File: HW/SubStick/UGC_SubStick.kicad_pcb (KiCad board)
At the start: 2 copper layers, 50.1 x 31 mm, 9 parts, among them J1 Conn_01x06_Pin, J2 503480-0640, SW1 GL18_SW, U1 GH39F (Hall SOT23), U2 GH39F (Hall SOT23)

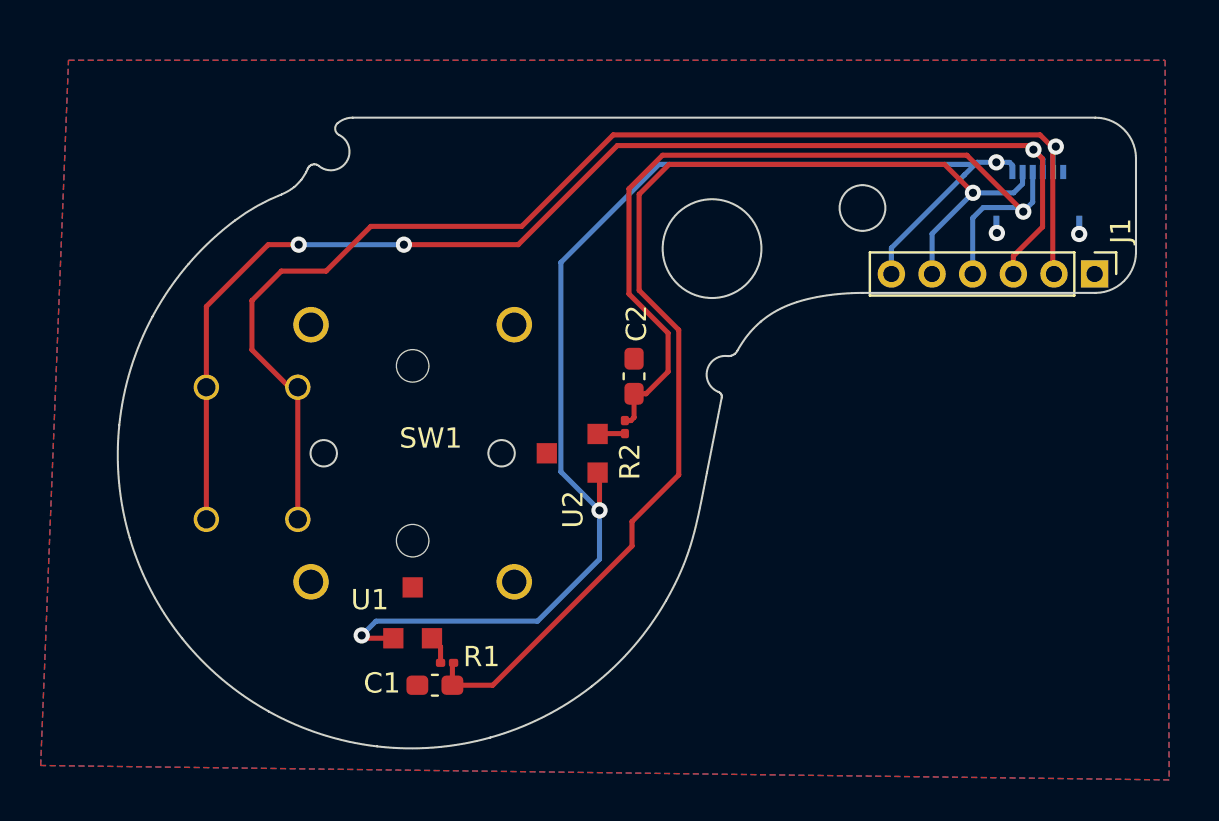
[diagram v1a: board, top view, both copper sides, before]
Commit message: R4 updates to hardware
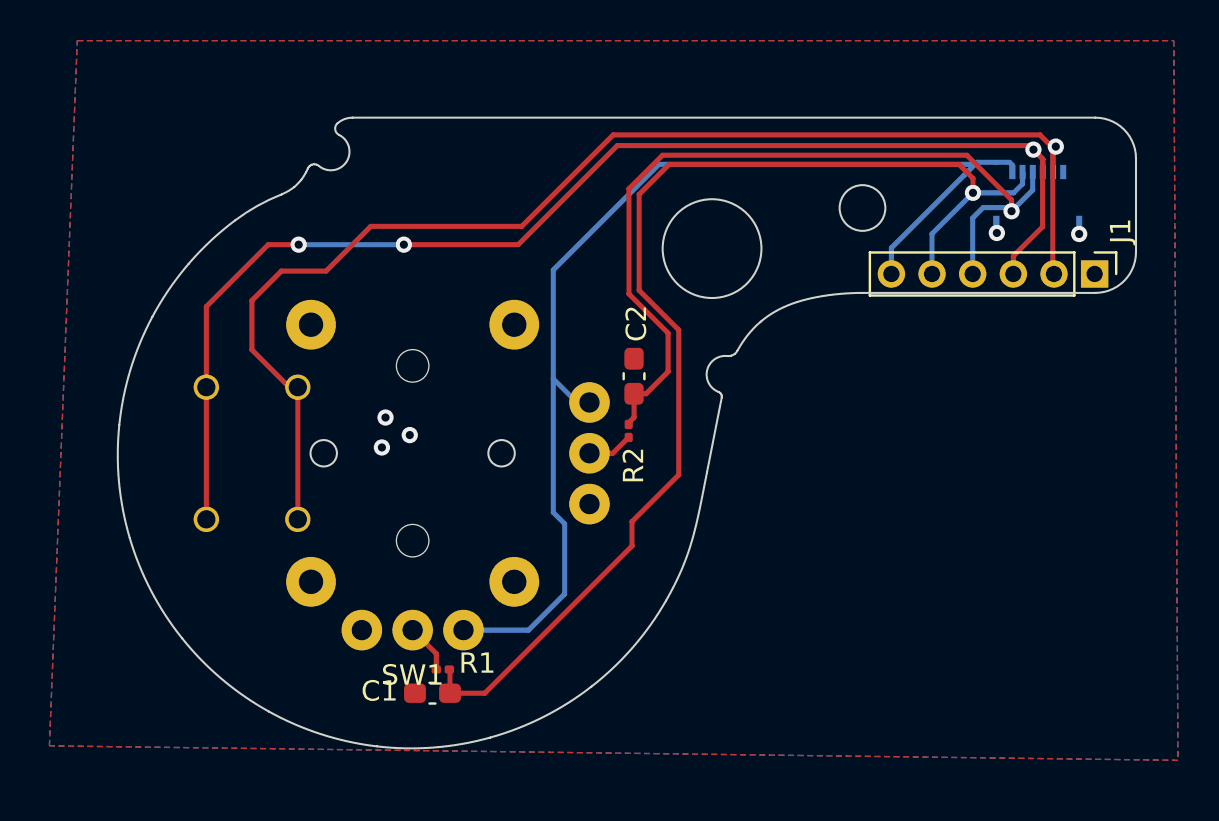
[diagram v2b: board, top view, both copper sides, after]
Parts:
- removed U1, U2: GH39F (Hall SOT23), hhl:GH39F
- SW1: footprint hhl:GL18 -> hhl:GL1807SYAE
- moved C1 0.41 mm to (248.2, 161.5)
- moved R1 0.39 mm to (248.7, 160.3)
- moved R2 0.27 mm to (257.8, 148.6)
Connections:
- R1 pad 1: Net-(U1-VOUT) -> Net-(SW1-X_OUT)
- R2 pad 1: Net-(U2-VOUT) -> Net-(SW1-Y_OUT)
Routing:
- net +3V3: track 64.0 -> 56.6 mm, vias 3 -> 0
- net Net-(SW1-X_OUT): track 0.00 -> 2.42 mm
- net Net-(SW1-Y_OUT): track 0.00 -> 2.25 mm
- net Net-(U1-VOUT): track 1.39 -> 0.00 mm
- net Net-(U2-VOUT): track 1.35 -> 0.00 mm
- net RX: track 57.5 -> 58.3 mm
- net RY: track 42.5 -> 41.8 mm
- net GND: track 0.72 -> 1.29 mm, vias 2 -> 5
